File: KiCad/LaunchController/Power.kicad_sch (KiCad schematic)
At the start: 39 parts, among them J1 DC_IN, J1 FROM_CONVERTER, J1 TO_CONVERTER, Q1 TJ8S06M3L, Q2 2SC3325-Y, Q3 TJ8S06M3L, U3 INA219BIDCNT, U5 INA219BIDCNT

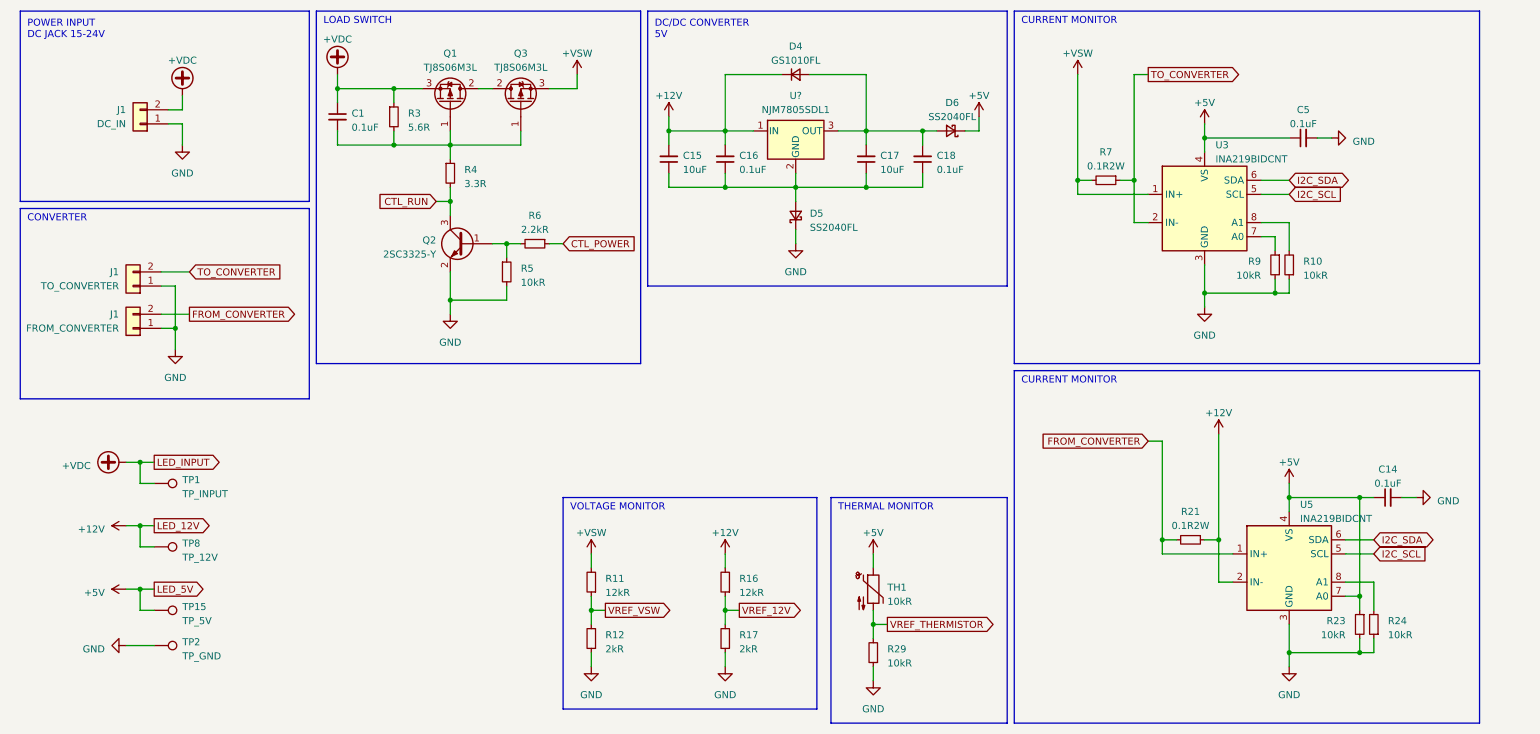
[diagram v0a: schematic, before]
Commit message: 選定部品を調整
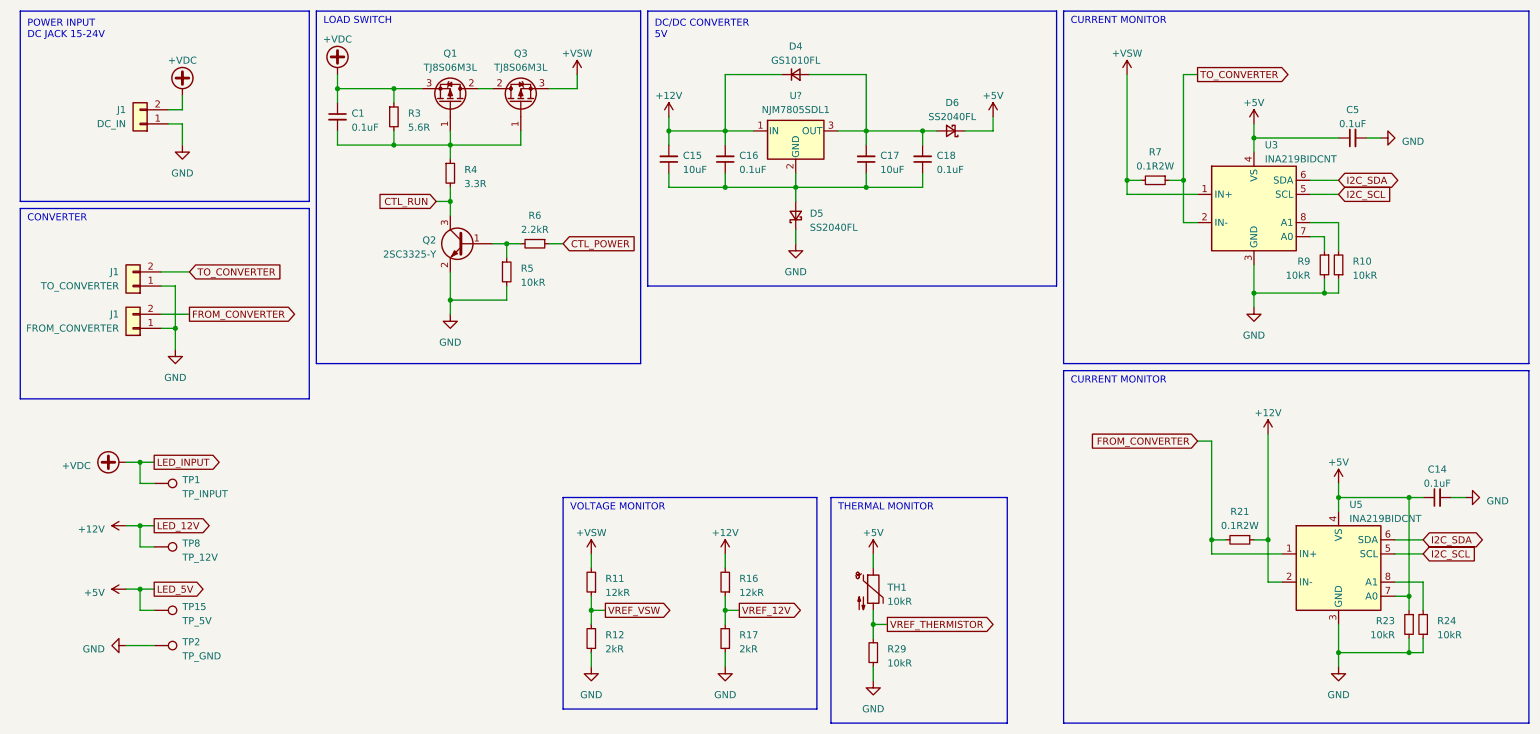
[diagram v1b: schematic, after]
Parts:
- C15, C17: footprint Capacitor_SMD:C_0603_1608Metric_Pad1.08x0.95mm_HandSolder -> Capacitor_SMD:C_1206_3216Metric_Pad1.33x1.80mm_HandSolder
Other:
- moved on the sheet: C14, C5, R10, R21, R23, R24, R7, R9, U3, U5
